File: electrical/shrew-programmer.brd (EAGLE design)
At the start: 50 x 50 mm, 9 parts, among them SW1 SWITCH-ROCKER-3PIN-2MNT, X1 PROG-JIG

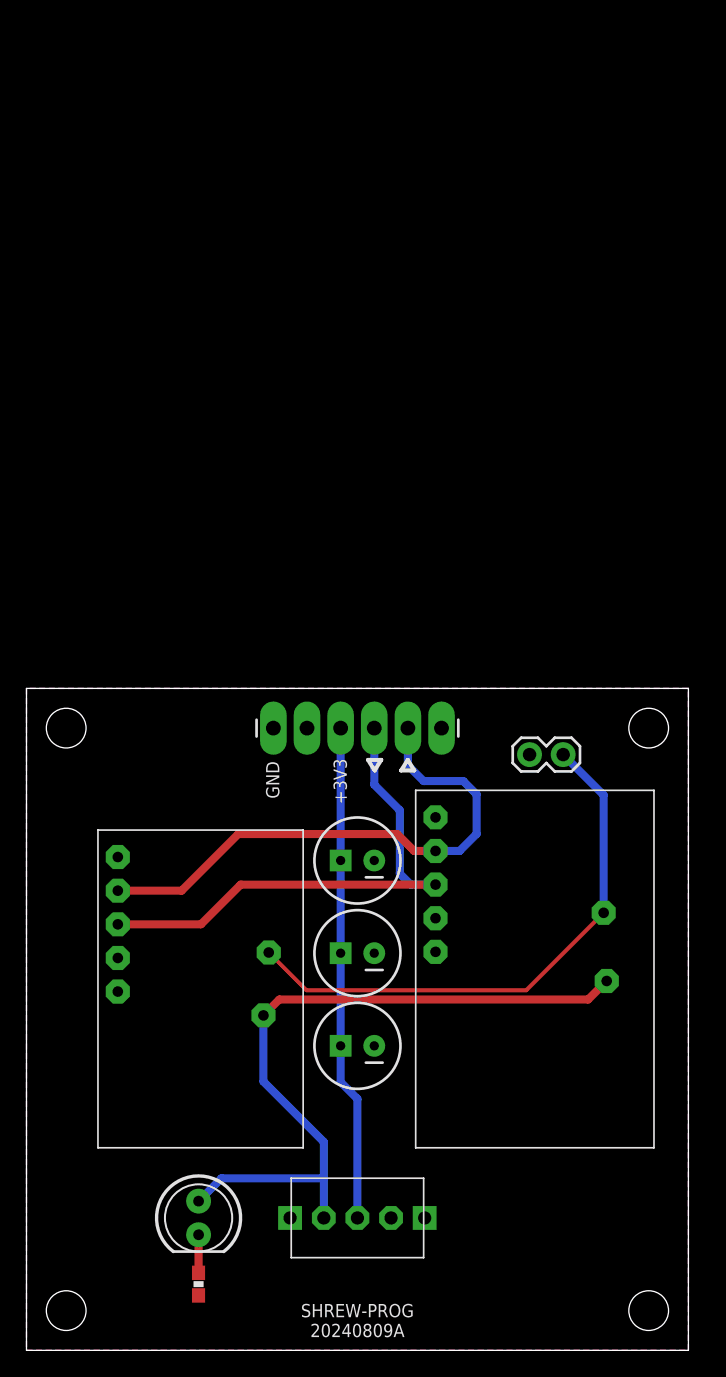
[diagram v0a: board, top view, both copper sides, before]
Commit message: another programmer PCB
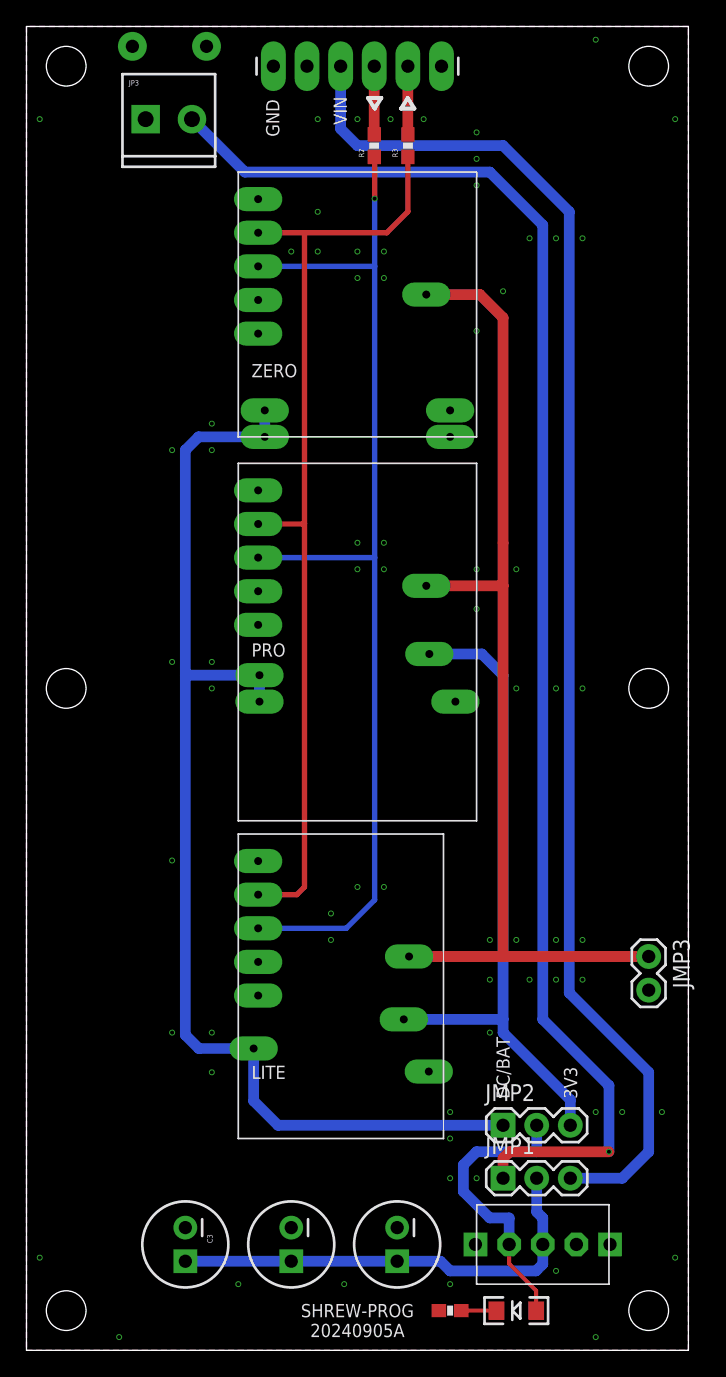
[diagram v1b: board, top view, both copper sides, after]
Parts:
- removed JP2: (no value), shrew-common:1X02
- added JMP1, JMP2: JUMPER-3PTH, shrew-common:1X03
- added JMP3: (no value), shrew-common:1X02
- added JP3: (no value), shrew-common:SCREWTERMINAL-3.5MM-2
- added R2, R3: (no value), shrew-common:0603-RES
- added X2: PROG-JIG-PRO, shrew-core:PROG-JIG-PRO
- added X3: PROG-JIG-ZERO, shrew-core:PROG-JIG-ZERO
- LED1: device shrew-common:LED5MM -> shrew-common:LED-1206
- X1: value PROG-JIG -> PROG-JIG-LITE; device shrew-core:JIG-PLACEMENTS -> shrew-core:PROG-JIG-LITE
- moved JP1 50.0 mm to (31.4, 97.0)
- moved C1 29.2 mm to (28.0, 8.00), turned to 270 degrees
- moved LED1 25.0 mm to (37.0, 3.00), turned to 180 degrees
- moved C2 22.6 mm to (20.0, 8.00), turned to 270 degrees
- moved C3 19.8 mm to (12.0, 8.00), turned to 270 degrees
- moved R1 19.1 mm to (32.0, 3.00), turned to 0 degrees
- moved SW1 14.1 mm to (39.0, 8.00)
- moved X1 10.6 mm to (16.0, 16.0)
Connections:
- removed net N$3: JP1.3, X1.RX1, X1.RX2
- new net 3V3: JMP2.3, X1.3V3, X2.3V3
- new net BOOT: JMP3.1, X1.BOOT, X2.BOOT, X3.BOOT
- new net PC-RX: R3.1, X1.TX, X2.TX, X3.TX
- new net PC-TX: R2.1, X1.RX, X2.RX, X3.RX
- new net V-DC: JMP1.1, JP3.2
- new net V-USB: JMP1.3, JP1.4
- new net VBAT: JMP2.1, X1.VBAT, X2.VBAT, X2.VBAT2, X3.VBAT, X3.VBAT2
- net GND: now also JMP3.2, JP3.1, X1.G, X1.G1, X2.G, X2.G1, X3.G, X3.G1, X3.G2; no longer JP2.1, X1.GND1, X1.GND2
- net N$1: now also JP1.3, R2.2; no longer JP1.2, X1.TX1, X1.TX2
- net N$2: now also JP1.2, R3.2; no longer LED1.A, SW1.1, X1.PWR1, X1.PWR2
- net N$4: now also JMP1.2; no longer JP1.4
- net N$5: now also LED1.C; no longer LED1.K
- net N$6: now also JMP2.2, LED1.A, SW1.1; no longer JP2.2, X1.BOOT1, X1.BOOT2
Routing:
- net V-DC: track 0.00 -> 111.6 mm, vias 0 -> 1
- net V-USB: track 0.00 -> 104.8 mm
- net VBAT: track 0.00 -> 89.3 mm
- net PC-TX: track 0.00 -> 83.4 mm, vias 0 -> 1
- net BOOT: track 0.00 -> 78.7 mm
- net PC-RX: track 0.00 -> 72.8 mm
- net 3V3: track 0.00 -> 49.8 mm
- net N$2: track 54.4 -> 5.15 mm
- net N$3: track 40.1 -> 0.00 mm, vias 0 -> 1
- net N$1: track 41.8 -> 5.15 mm
- net N$6: track 42.1 -> 22.1 mm
- net N$4: track 37.5 -> 34.2 mm
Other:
- board size 50 x 50 mm -> 50 x 100 mm
- board text added: "3V3"
- board text added: "DC/BAT"
- board text added: "LITE"
- board text added: "PRO"
- board text added: "SHREW-PROG 20240905A"
- board text added: "VIN"
- board text added: "ZERO"
- board text removed: "+3V3"
- board text removed: "SHREW-PROG 20240809A"
